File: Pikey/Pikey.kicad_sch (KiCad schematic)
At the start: 58 parts, among them J1 DX07P024AJ1R1500, J2 Conn_01x03, J3 Micro_SD_Card_Det2, SW1 CK_KMS2xxG, SW2 CK_KMS2xxG, U1 RP2350B, U2 NCP1117-3.3_SOT223, U3 W25Q128JVS, Y1 ABM8-272-T3

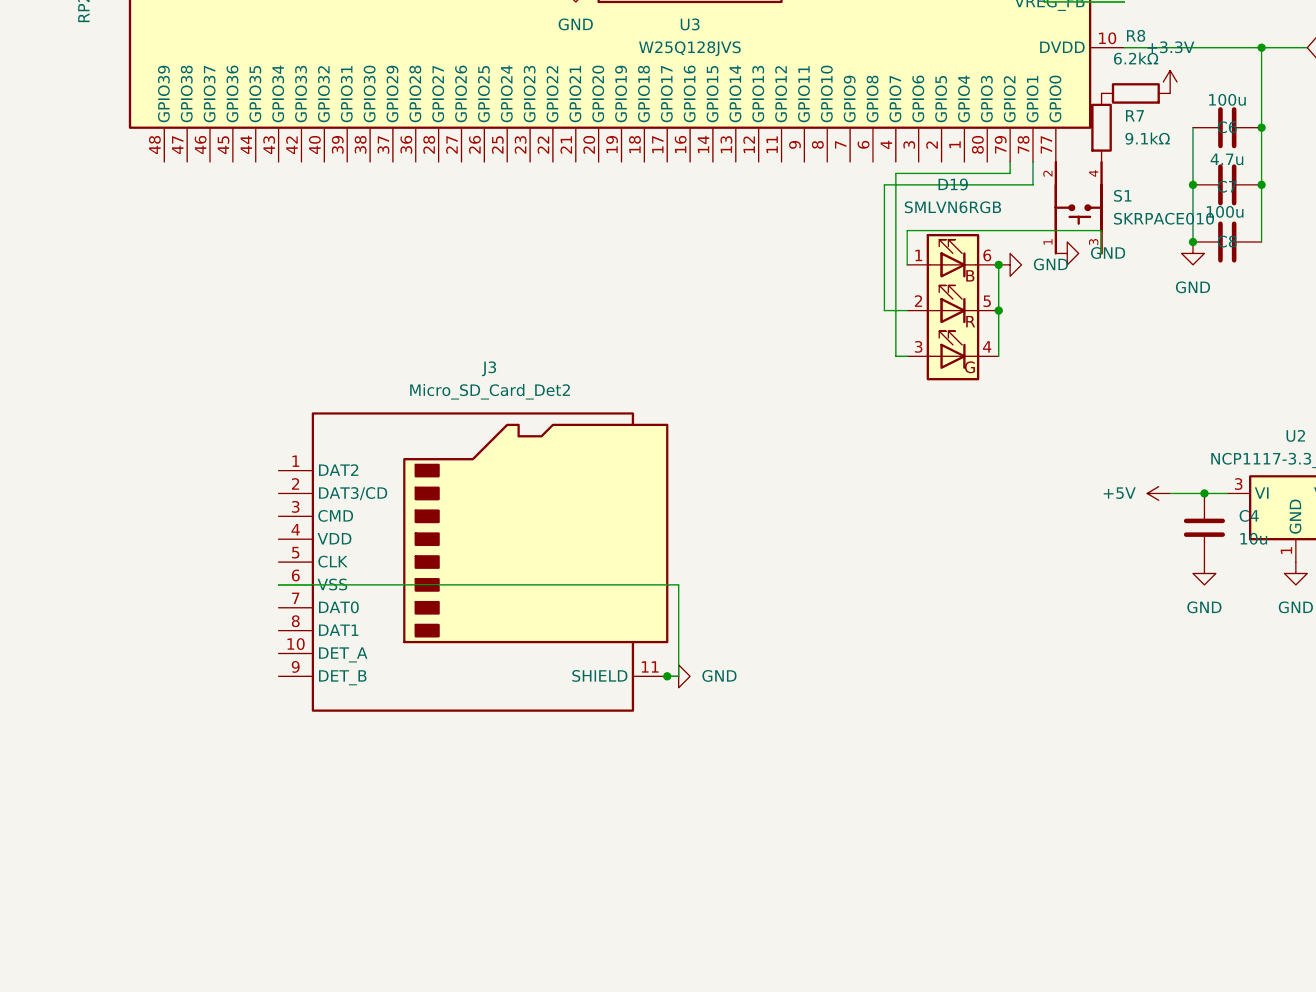
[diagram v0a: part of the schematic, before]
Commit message: 13th April update
added the nRF8001
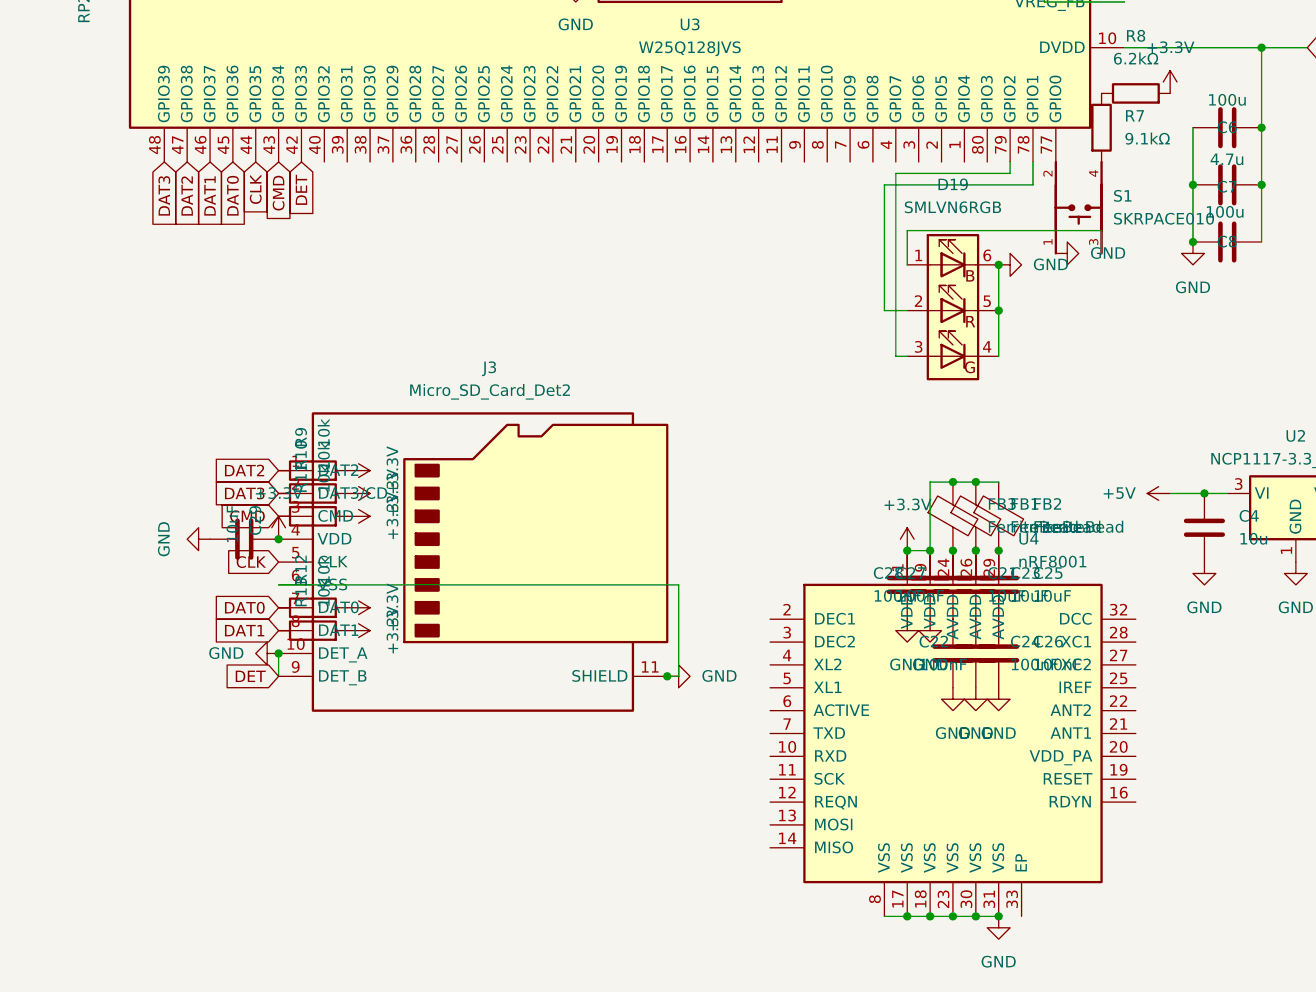
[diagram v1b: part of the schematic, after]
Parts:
- added C21, C23, C25, C29: 10uF, Capacitor_SMD:C_0402_1005Metric, symbol Device:C
- added C22, C24, C26, C27, C28: 100nF, Capacitor_SMD:C_0402_1005Metric, symbol Device:C
- added FB1, FB2, FB3: FerriteBead, Inductor_SMD:L_0402_1005Metric, symbol Device:FerriteBead
- added R10, R11, R12, R13, R9: 10k, Resistor_SMD:R_0201_0603Metric, symbol Device:R
- added U4: nRF8001, Package_DFN_QFN:QFN-32-1EP_5x5mm_P0.5mm_EP3.45x3.45mm, symbol RF_Bluetooth:nRF8001
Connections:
- net +3.3V: now also J3.4 (VDD), C27.1, C28.1, C29.1, FB1.1, FB2.1, FB3.1, R10.2, R11.2, R12.2, R13.2, R9.2, U4.1 (VDD), U4.9 (VDD)
- net GND: now also J3.10 (DET_A), J3.9 (DET_B), U1.42 (GPIO33), C22.2, C24.2, C26.2, C27.2, C28.2, C29.2, U4.17 (VSS), U4.18 (VSS), U4.23 (VSS), U4.30 (VSS), U4.31 (VSS), U4.8 (VSS)
- net DAT2: now reaches J3.1 (DAT2)
- net DAT2: now also U1.47 (GPIO38), R9.1
- net DAT3: now reaches J3.2 (DAT3/CD)
- net DAT3: now also U1.48 (GPIO39), R10.1
- net CMD: now reaches J3.3 (CMD)
- net CMD: now also U1.43 (GPIO34), R11.1
- net CLK: now reaches J3.5 (CLK)
- net CLK: now also U1.44 (GPIO35)
- net DAT0: now reaches J3.7 (DAT0)
- net DAT0: now also U1.45 (GPIO36), R12.1
- net DAT1: now reaches J3.8 (DAT1)
- net DAT1: now also U1.46 (GPIO37), R13.1
- new net: C21.1, FB3.2, U4.24 (AVDD)
- new net: C21.2, C22.1
- new net: C23.2, C24.1
- new net: C25.2, C26.1
- new net: C25.1, FB2.2, U4.29 (AVDD)
- new net: C23.1, FB1.2, U4.26 (AVDD)
